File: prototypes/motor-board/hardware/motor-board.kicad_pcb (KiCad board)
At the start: 2 copper layers, 1 part

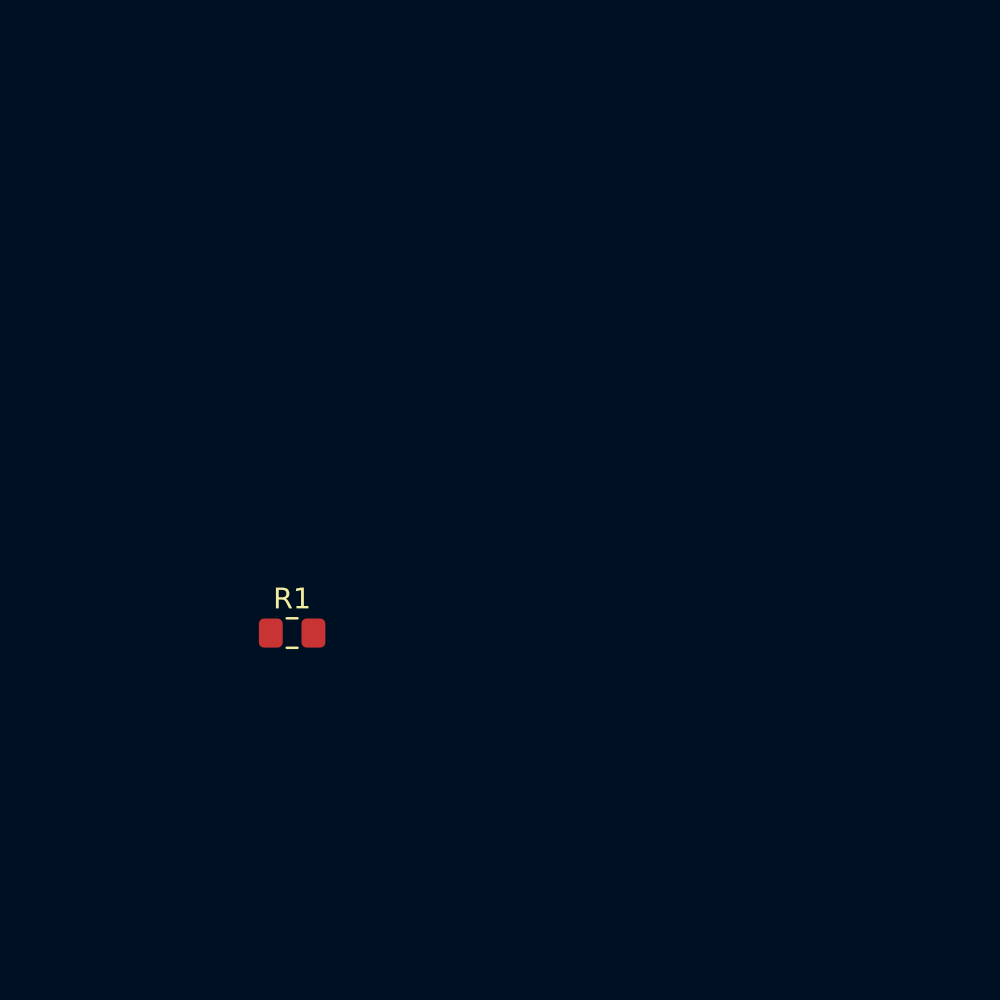
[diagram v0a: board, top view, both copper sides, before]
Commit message: Finish up motor board schematic; start on layout
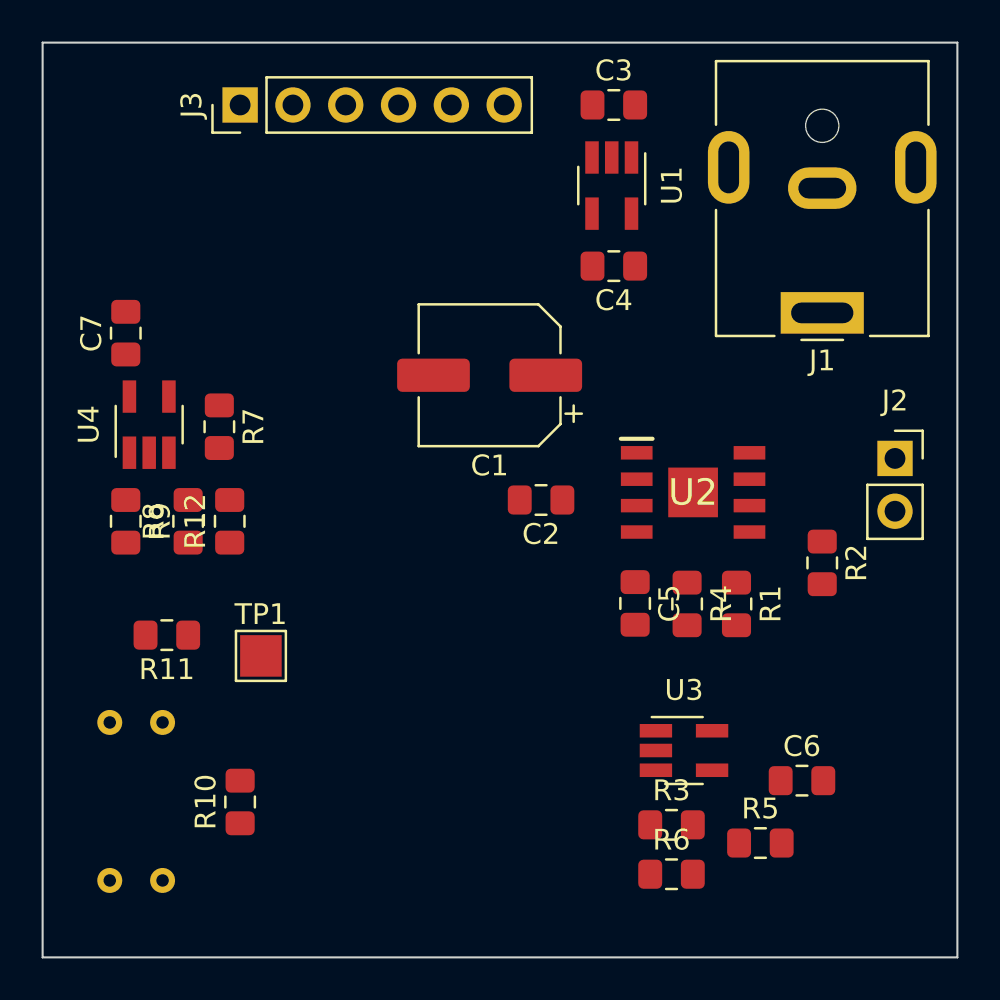
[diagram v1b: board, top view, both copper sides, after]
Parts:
- added C1: 100U, mini-mapper:CP_Elec_6.3x7.7, F.Cu at (128.5, 95.0)
- added C2: 0.1U, mini-mapper:C_0805, F.Cu at (131.0, 101.0)
- added C3: 1U, mini-mapper:C_0805, F.Cu at (134.5, 82.0)
- added C4: 1U, mini-mapper:C_0805, F.Cu at (134.5, 89.8)
- added C5: 0.1U, mini-mapper:C_0805, F.Cu at (135.5, 106.0)
- added C6: 0.1U, mini-mapper:C_0805, F.Cu at (143.5, 114.5)
- added C7: 0.1U, mini-mapper:C_0805, F.Cu at (111.0, 93.0)
- added J1: PJ-063AH, mini-mapper:BarrelJack_CUI_PJ-063AH_Horizontal, F.Cu at (144.5, 92.0)
- added J2: Conn_01x02, mini-mapper:PinSocket_1x02_P2.54mm_Vertical, F.Cu at (148.0, 99.0)
- added J3: PinHeader_01x06, mini-mapper:PinHeader_1x06_P2.54mm_Vertical, F.Cu at (116.5, 82.0)
- added R10: 82, mini-mapper:R_0805, F.Cu at (116.5, 115.5)
- added R11: 5.7K, mini-mapper:R_0805, F.Cu at (113.0, 107.5)
- added R12: 1K, mini-mapper:R_0805, F.Cu at (116.0, 102.0)
- added R2: 400m, mini-mapper:R_0805, F.Cu at (144.5, 104.0)
- added R3: 12K, mini-mapper:R_0805, F.Cu at (137.2, 116.6)
- added R4: 2K, mini-mapper:R_0805, F.Cu at (138.0, 106.0)
- added R5: 330K, mini-mapper:R_0805, F.Cu at (141.5, 117.5)
- added R6: 220K, mini-mapper:R_0805, F.Cu at (137.2, 119.0)
- added R7: 32K, mini-mapper:R_0805, F.Cu at (115.5, 97.5)
- added R8: 1K, mini-mapper:R_0805, F.Cu at (114.0, 102.0)
- added R9: 1K, mini-mapper:R_0805, F.Cu at (111.0, 102.0)
- added TP1: TestPoint, mini-mapper:TestPoint_Pad_2.0x2.0mm, F.Cu at (117.5, 108.5)
- added U1: TLV70245_SOT23-5, mini-mapper:SOT-23-5, F.Cu at (134.4, 85.9)
- added U2: TB67H450FNG, mini-mapper:SOIC127P600X175-9N, F.Cu at (138.3, 100.6)
- added U3: TLV9051, mini-mapper:SOT-23-5, F.Cu at (137.8, 113.0)
- added U4: LMV331, mini-mapper:SOT-23-5, F.Cu at (112.1, 97.4)
- added U5: TCST1202, mini-mapper:TCST1202, B.Cu at (111.5, 115.5)
- R1: value R -> 7K
- moved R1 21.4 mm to (140.4, 106.0), turned to 270 degrees
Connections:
- R1 pad 1: Net-(R1-Pad1) -> VM
- R1 pad 2: Net-(R1-Pad1) -> /Vref
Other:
- board outline added: 44 x 44 mm

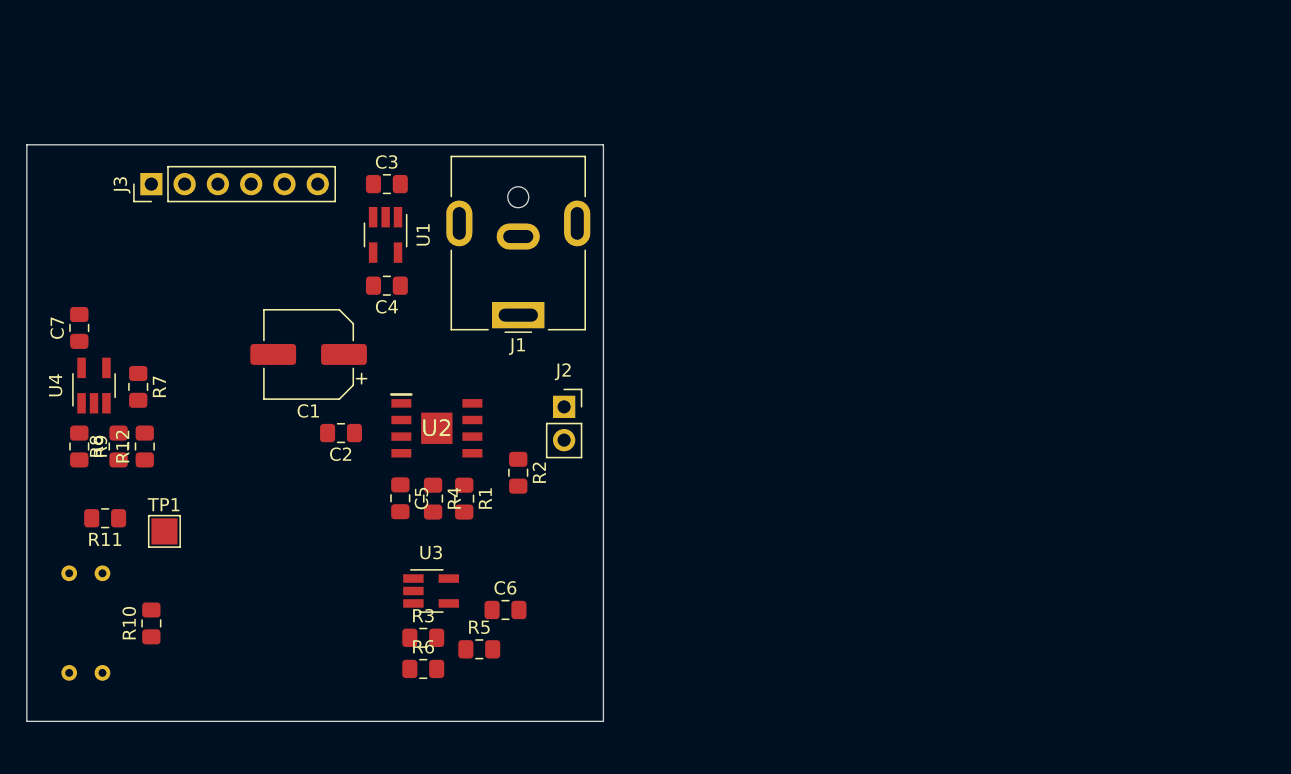
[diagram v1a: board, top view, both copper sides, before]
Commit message: Missed some changes...
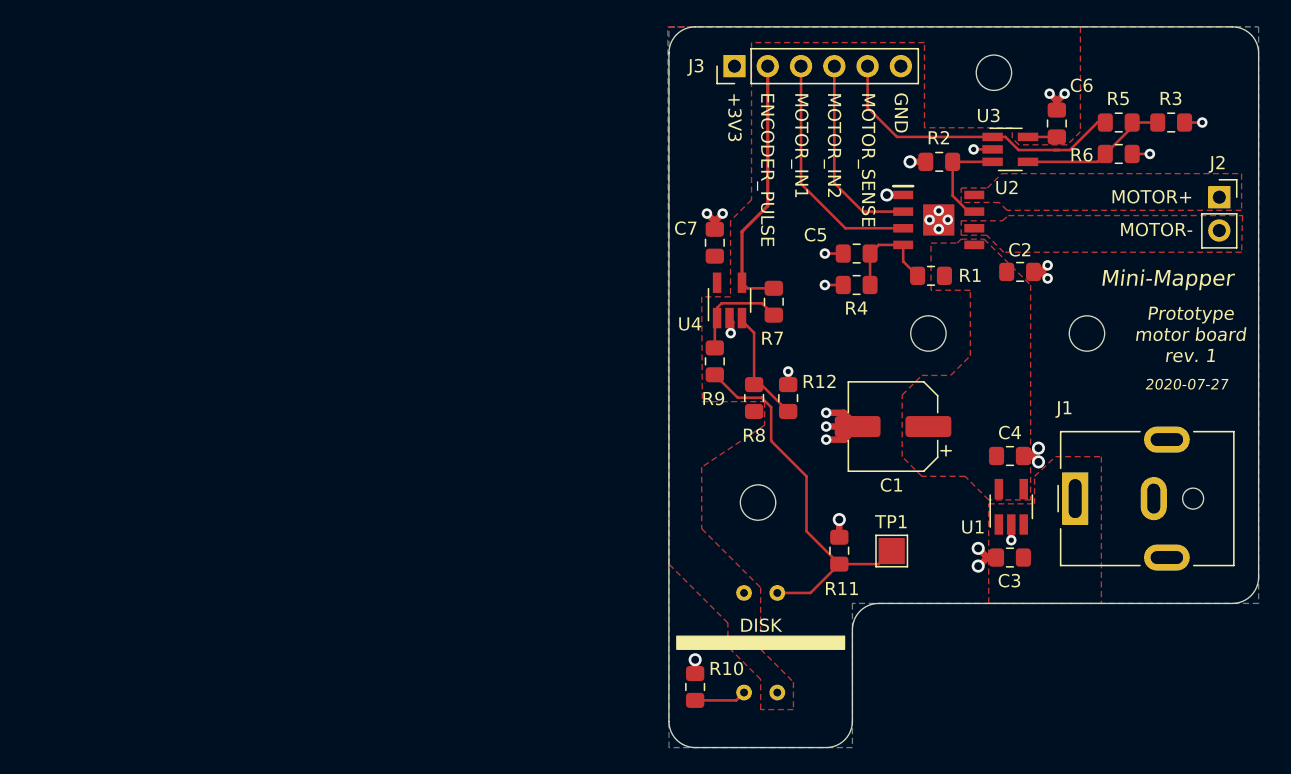
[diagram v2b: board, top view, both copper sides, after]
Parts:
- added H1: MountingHole, mini-mapper:MountingHole_2.7mm_M2.5, F.Cu at (175.8, 93.4)
- added H2: MountingHole, mini-mapper:MountingHole_2.7mm_M2.5, F.Cu at (162.8, 106.3)
- added H3: MountingHole, mini-mapper:MountingHole_2.7mm_M2.5, F.Cu at (187.9, 93.4)
- added H4: MountingHole, mini-mapper:MountingHole_2.7mm_M2.5, F.Cu at (180.8, 73.5)
- R1: value 7K -> 56K
- R11: value 5.7K -> 5.6K
- R4: value 2K -> 16K
- R7: value 32K -> 240K
- R9: value 1K -> 7.5K
- moved R3 69.3 mm to (194.3, 77.3), turned to 180 degrees
- moved R6 66.0 mm to (190.3, 79.7), turned to 180 degrees
- moved R5 63.2 mm to (190.3, 77.3), turned to 180 degrees
- moved C6 56.1 mm to (185.6, 77.4), turned to 90 degrees
- moved R11 56.1 mm to (169.0, 110.0), turned to 90 degrees
- moved U3 55.6 mm to (182.1, 79.3)
- moved TP1 55.5 mm to (173.0, 110.0)
- moved C3 55.4 mm to (182.0, 110.5), turned to 180 degrees
- moved C2 53.3 mm to (182.8, 88.7), turned to 0 degrees
- moved J2 52.5 mm to (198.0, 83.0)
- moved U1 52.1 mm to (182.1, 106.6), turned to 90 degrees
- moved U5 51.5 mm to (163.0, 117.0)
- moved C4 49.3 mm to (182.0, 102.8), turned to 0 degrees
- moved R12 49.2 mm to (165.1, 98.3)
- moved C7 48.9 mm to (159.5, 86.5)
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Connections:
- net Net-(C3-Pad1) renamed /VIN
- net Net-(J2-Pad1) renamed /MOTOR1
- net Net-(J2-Pad2) renamed /MOTOR2
- J3 pad 3: /MOTOR_SENSE -> /MOTOR_IN1
- J3 pad 4: /MOTOR_IN1 -> /MOTOR_IN2
- J3 pad 5: /MOTOR_IN2 -> /MOTOR_SENSE
- U2 pad 9: (no net) -> GND
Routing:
- net GND: track 0.00 -> 36.5 mm, vias 0 -> 29
- net /Vphoto: track 0.00 -> 29.5 mm
- net /MOTOR_SENSE: track 0.00 -> 23.9 mm
- net /ENCODER_PULSE: track 0.00 -> 19.9 mm
- net /MOTOR_IN1: track 0.00 -> 18.2 mm
- net /MOTOR_IN2: track 0.00 -> 15.1 mm
- net Net-(R3-Pad2): track 0.00 -> 11.3 mm
- net Net-(R12-Pad1): track 0.00 -> 8.91 mm
- net /Vref: track 0.00 -> 8.01 mm
- net Net-(R7-Pad2): track 0.00 -> 7.98 mm
- net /Isense+: track 0.00 -> 7.79 mm
- net Net-(R10-Pad1): track 0.00 -> 3.98 mm
- net +3V3: track 0.00 -> 2.20 mm
- added copper zone on F.Cu, net +3V3
- added copper zone on F.Cu, net /MOTOR1
- added copper zone on F.Cu, net /MOTOR2
- added copper zone on F.Cu, net /VIN
- added copper zone on B.Cu, net GND
- added copper zone on F.Cu, net VM
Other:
- board size 44 x 44 mm -> 45 x 55 mm
- board text added: "+3V3"
- board text added: "2020-07-27"
- board text added: "DISK"
- board text added: "ENCODER_PULSE"
- board text added: "GND"
- board text added: "MOTOR+"
- board text added: "MOTOR-"
- board text added: "MOTOR_IN1"
- board text added: "MOTOR_IN2"
- board text added: "MOTOR_SENSE"
- board text added: "Mini-Mapper"
- board text added: "Prototype motor board rev. 1"
